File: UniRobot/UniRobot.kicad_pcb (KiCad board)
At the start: 2 copper layers, 53.5 x 65.5 mm, 15 parts, among them J1 Conn_01x01_Socket, J2 Conn_01x01_Socket, J3 Conn_01x02_Socket, K1 G5V-1-DC5, Q1 BSS138, U1 RFM69HW

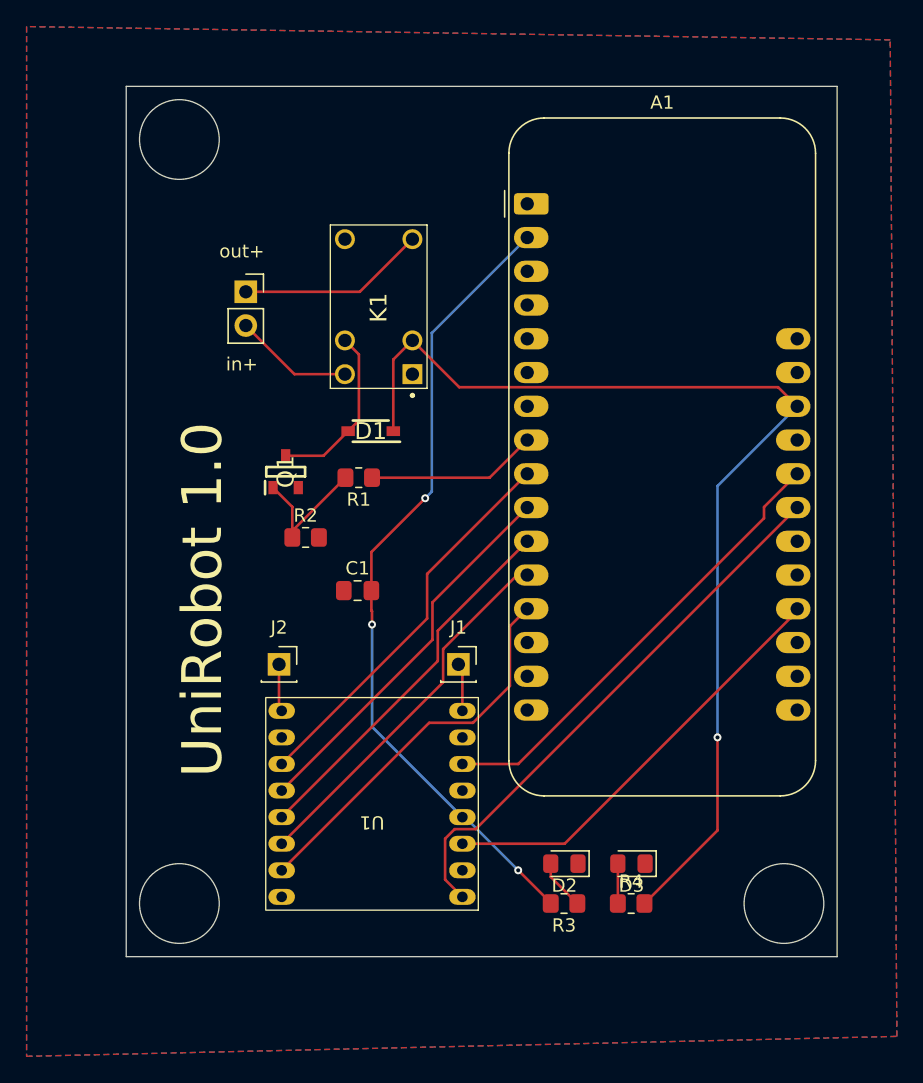
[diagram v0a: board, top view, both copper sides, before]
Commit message: pcb
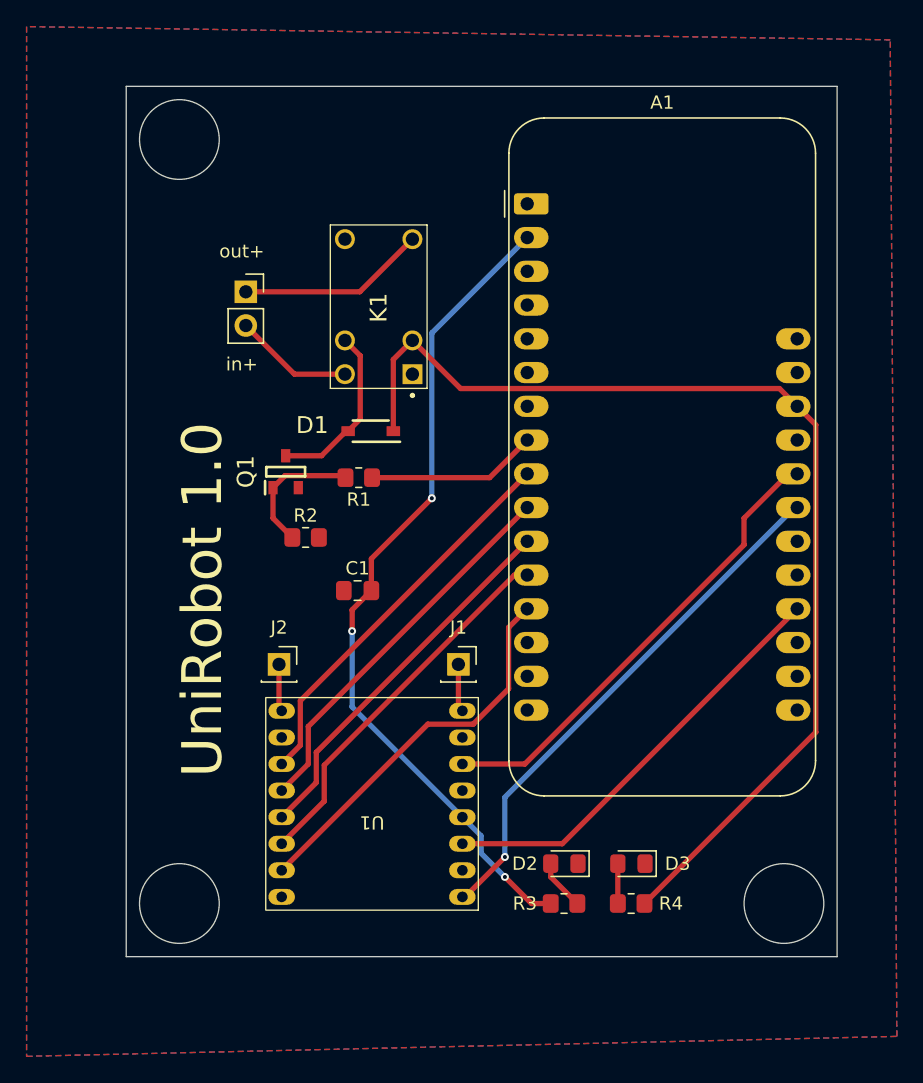
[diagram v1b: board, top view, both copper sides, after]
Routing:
- net +3.3V: track 60.7 -> 62.6 mm
- net DIO2: track 41.7 -> 40.0 mm, vias 0 -> 1
- net Net-(A1-USB): track 80.6 -> 81.8 mm, vias 1 -> 0
- net Net-(J3-Pin_1): track 14.2 -> 14.9 mm
- net DIO3: track 34.7 -> 35.4 mm
